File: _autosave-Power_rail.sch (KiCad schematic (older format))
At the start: 9 parts, among them J3 Conn_01x08_Male, J4 Conn_01x08_Male, J5 Conn_01x08_Male, J6 Conn_01x02_Male, J7 Conn_01x03_Male, J8 Conn_01x02_Male, Q1 2N3904

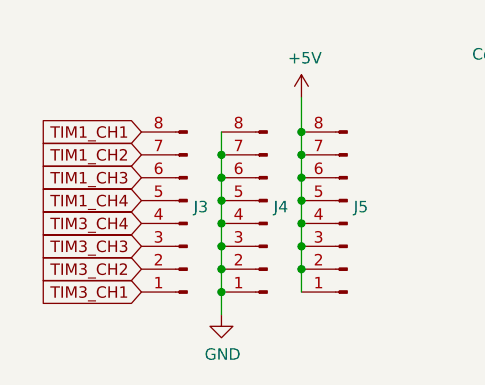
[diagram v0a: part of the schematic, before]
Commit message: a
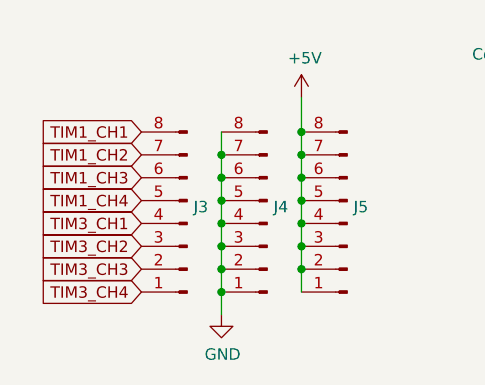
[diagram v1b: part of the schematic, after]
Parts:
- J7: footprint Connector_JST:JST_PH_B3B-PH-K_1x03_P2.00mm_Vertical -> Connector_JST:JST_SH_BM03B-SRSS-TB_1x03-1MP_P1.00mm_Vertical
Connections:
- net TIM3_CH1: now also J3.4 (Pin_4); no longer J3.1 (Pin_1)
- net TIM3_CH2: now also J3.3 (Pin_3); no longer J3.2 (Pin_2)
- net TIM3_CH3: now also J3.2 (Pin_2); no longer J3.3 (Pin_3)
- net TIM3_CH4: now also J3.1 (Pin_1); no longer J3.4 (Pin_4)
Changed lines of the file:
@@
 F 0 "J7" H 6672 4028 50  0000 R CNN
 F 1 "Conn_01x03_Male" H 6672 4073 50  0001 R CNN
-F 2 "Connector_JST:JST_PH_B3B-PH-K_1x03_P2.00mm_Vertical" H 6700 4050 50  0001 C CNN
+F 2 "Connector_JST:JST_SH_BM03B-SRSS-TB_1x03-1MP_P1.00mm_Vertical" H 6700 4050 50  0001 C CNN
 F 3 "~" H 6700 4050 50  0001 C CNN
 	1    6700 4050
@@
 	1    0    0    -1
 $EndComp
+Text GLabel 3500 4150 0    50   Input ~ 0
+TIM3_CH2
 Text GLabel 3500 4250 0    50   Input ~ 0
-TIM3_CH2
-Text GLabel 3500 4150 0    50   Input ~ 0
 TIM3_CH3
 Wire Wire Line
@@
 	-1   0    0    1
 $EndComp
+Text GLabel 3500 4050 0    50   Input ~ 0
+TIM3_CH1
 Text GLabel 3500 4350 0    50   Input ~ 0
-TIM3_CH1
-Text GLabel 3500 4050 0    50   Input ~ 0
 TIM3_CH4
 Text GLabel 3500 3650 0    50   Input ~ 0
